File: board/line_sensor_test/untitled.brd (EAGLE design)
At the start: 100 x 100 mm, 93 parts, among them U1 74HC4067SSOP-24, U2 74HC4067SSOP-24

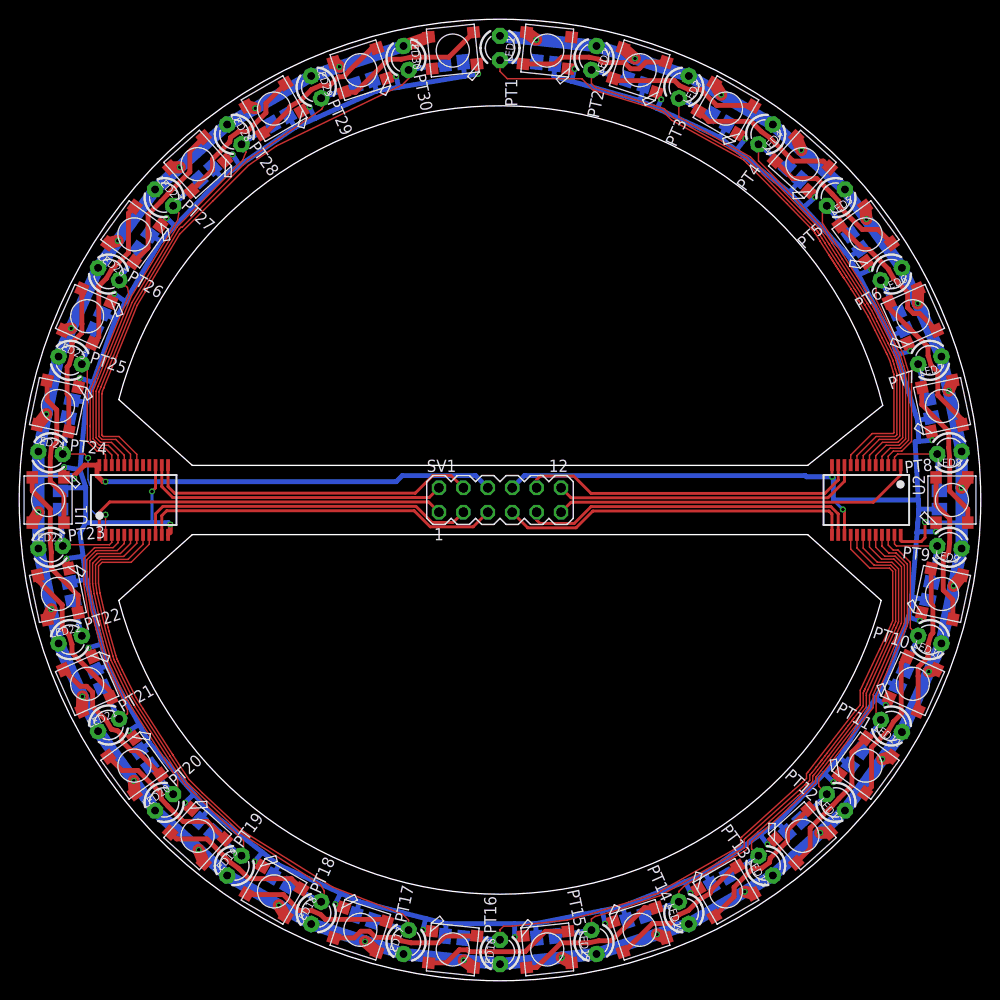
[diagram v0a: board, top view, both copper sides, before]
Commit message: encorder & linesensor
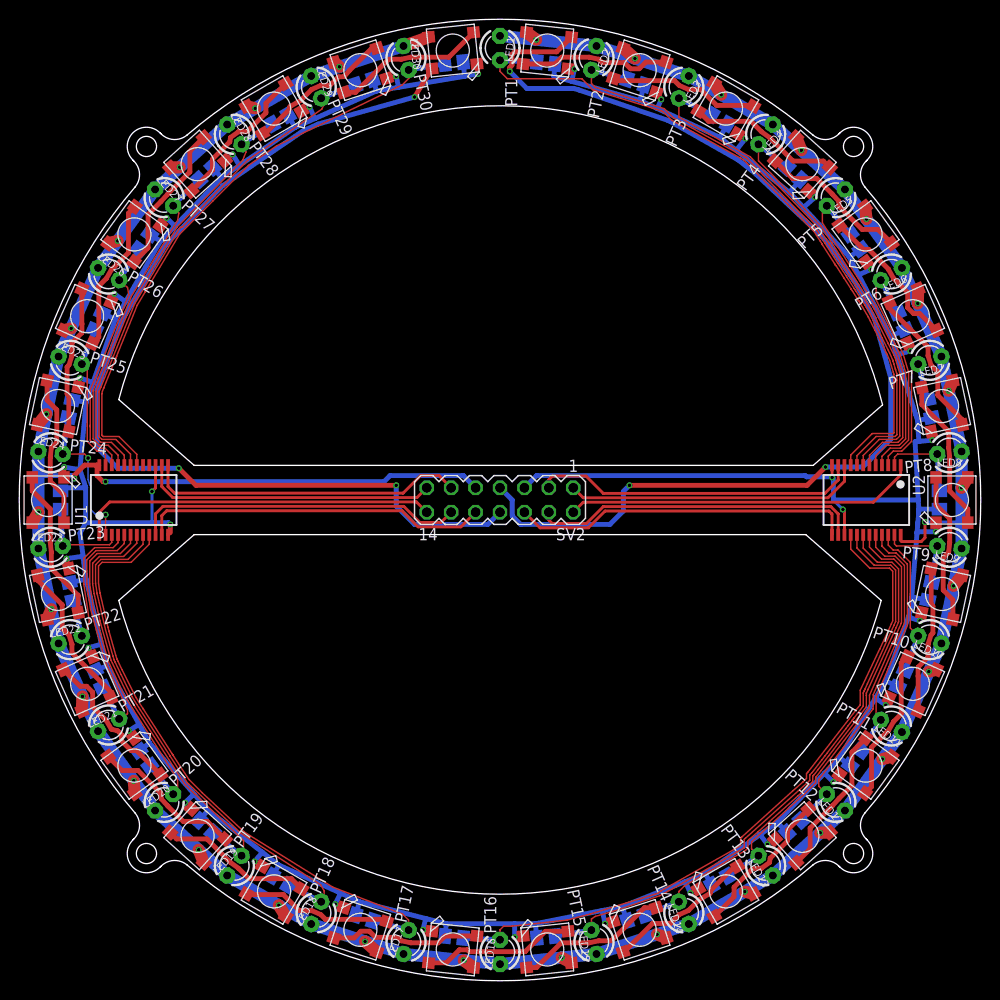
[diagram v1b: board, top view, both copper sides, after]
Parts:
- removed SV1: (no value), con-lstb:MA06-2
- added SV2: (no value), con-lstb:MA07-2
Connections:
- removed net N$60: LED1.4-DIN
- new net LED_IN: LED1.4-DIN, SV2.7
- new net LED_OUT: LED30.2-DOUT, SV2.8
- net AIN0: now also SV2.14; no longer SV1.1
- net AIN1: now also SV2.2; no longer SV1.11
- net GND: now also SV2.5; no longer SV1.8
- net N$10: now also SV2.6; no longer SV1.7
- net N$11: now also SV2.4; no longer SV1.9
- net N$13: now also SV2.3; no longer SV1.10
- net N$14: now also SV2.1; no longer SV1.12
- net N$15: now also SV2.10; no longer SV1.5
- net N$16: now also SV2.12; no longer SV1.3
- net N$8: now also SV2.13; no longer SV1.2
- net N$9: now also SV2.11; no longer SV1.4
- net VCC: now also SV2.9; no longer SV1.6
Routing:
- net LED_IN: track 0.00 -> 117.7 mm, vias 0 -> 3
- net LED_OUT: track 0.00 -> 104.0 mm, vias 0 -> 3
- net A1: track 76.1 -> 73.2 mm
- net AIN0: track 38.7 -> 37.3 mm
- net N$8: track 31.9 -> 30.7 mm
- net N$16: track 35.7 -> 34.4 mm
- net N$13: track 35.2 -> 34.0 mm
- net N$14: track 32.3 -> 31.0 mm
- net N$9: track 34.5 -> 33.2 mm
- net N$15: track 37.4 -> 36.2 mm
- net N$11: track 35.5 -> 34.3 mm
- net N$10: track 37.0 -> 35.7 mm
- net AIN1: track 37.9 -> 36.7 mm
- net VCC: track 400.2 -> 398.9 mm
- net GND: track 456.1 -> 454.9 mm
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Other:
- outline, holes or cut-outs redrawn
